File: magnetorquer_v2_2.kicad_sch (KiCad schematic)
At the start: 13 parts, among them U1 MSP430FR5994IPN, Y1 Crystal

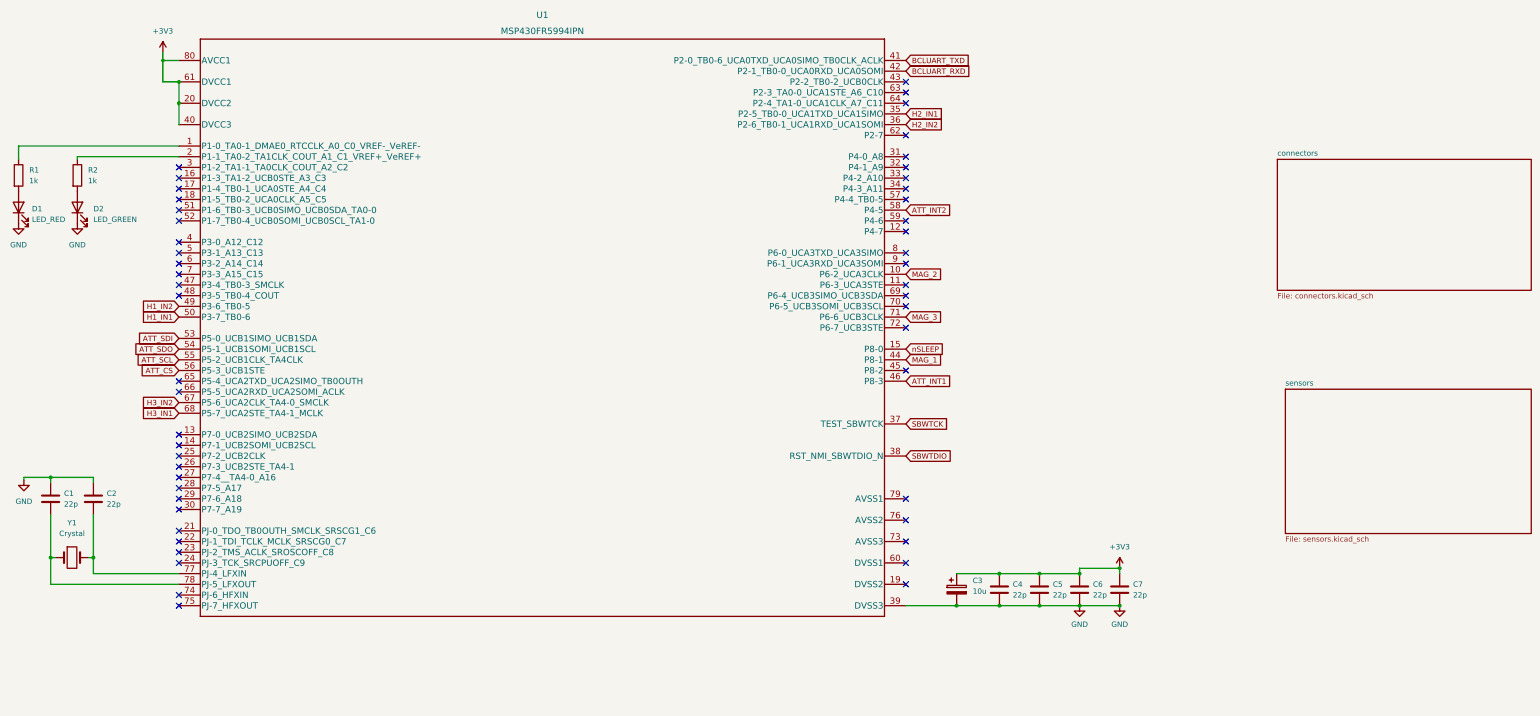
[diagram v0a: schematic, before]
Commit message: new uc
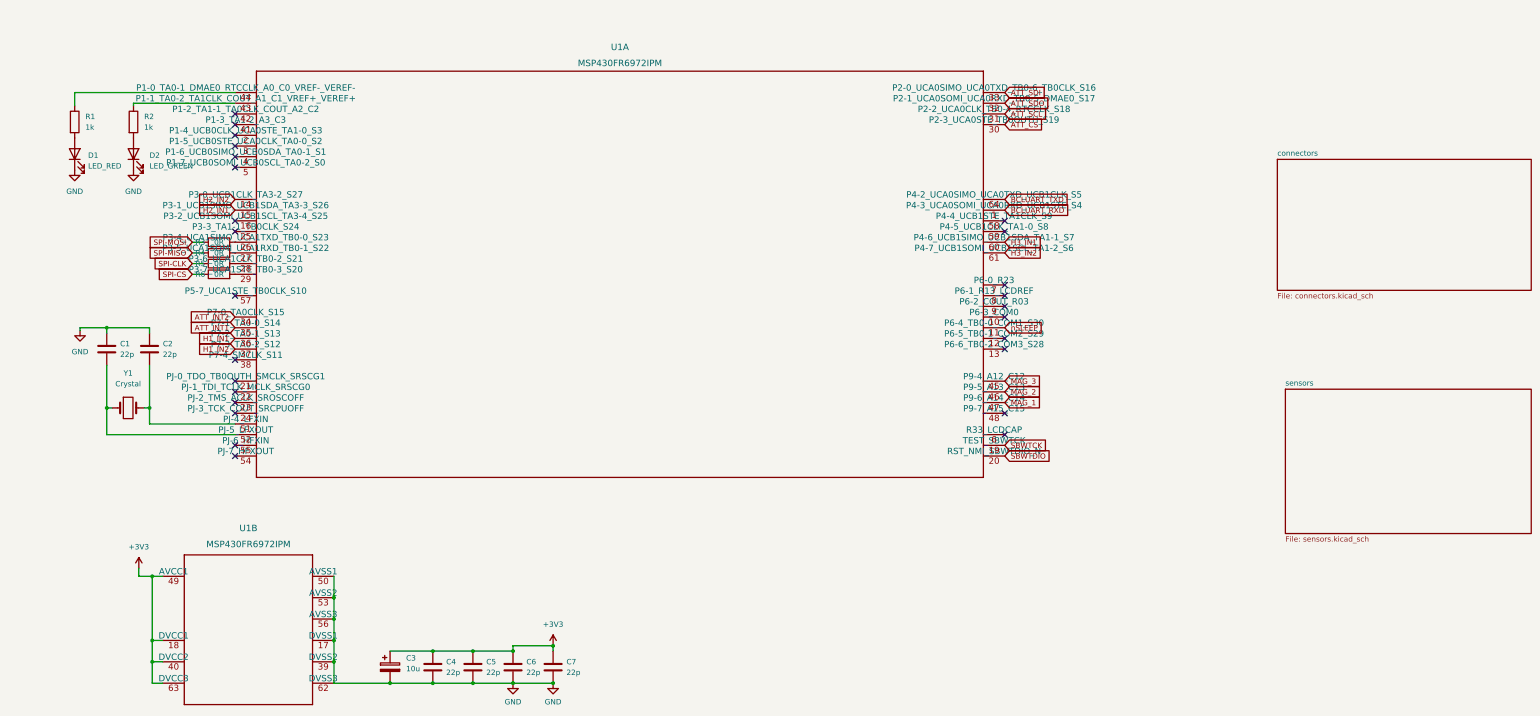
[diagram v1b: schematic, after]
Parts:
- removed U1: MSP430FR5994IPN, magnetorquer:MSP430FR5994IPN, symbol MSP430FR5994IPN:MSP430FR5994IPN
- added R3, R4, R5, R6: 0R, Resistor_SMD:R_0805_2012Metric, symbol Device:R
- added U1: MSP430FR6972IPM, magnetorquer:MSP430FR6972IPM, symbol MSP430FR6972IPM-B:MSP430FR6972IPM
- C3: footprint Capacitor_SMD:C_0805_2012Metric -> Capacitor_Tantalum_SMD:CP_EIA-3216-18_Kemet-A
- D1, D2: footprint LED_SMD:LED_0805_2012Metric -> LED_SMD:LED_0603_1608Metric
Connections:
- net +3V3: now also U1.18 (DVCC1), U1.40 (DVCC2), U1.49 (AVCC1), U1.63 (DVCC3)
- net ATT_CS: now also U1.30 (P2-3_UCA0STE_TB0OUTH_S19)
- net ATT_INT1: now also U1.35 (P7-1_TA0-0_S14)
- net ATT_INT2: now also U1.34 (P7-0_TA0CLK_S15)
- net ATT_SCL: now also U1.31 (P2-2_UCA0CLK_TB0-4_RTCCLK_S18)
- net ATT_SDI: now also U1.33 (P2-0_UCA0SIMO_UCA0TXD_TB0-6_TB0CLK_S16)
- net ATT_SDO: now also U1.32 (P2-1_UCA0SOMI_UCA0RXD_TB0-5_DMAE0_S17)
- net BCLUART_RXD: now also U1.1 (P4-3_UCA0SOMI_UCA0RXD_UCB1STE_S4)
- net BCLUART_TXD: now also U1.64 (P4-2_UCA0SIMO_UCA0TXD_UCB1CLK_S5)
- net GND: now also U1.17 (DVSS1), U1.39 (DVSS2), U1.50 (AVSS1), U1.53 (AVSS2), U1.56 (AVSS3), U1.62 (DVSS3)
- net H1_IN1: now also U1.36 (P7-2_TA0-1_S13)
- net H1_IN2: now also U1.37 (P7-3_TA0-2_S12)
- net H2_IN1: now also U1.15 (P3-1_UCB1SIMO_UCB1SDA_TA3-3_S26)
- net H2_IN2: now also U1.14 (P3-0_UCB1CLK_TA3-2_S27)
- net H3_IN1: now also U1.60 (P4-6_UCB1SIMO_UCB1SDA_TA1-1_S7)
- net H3_IN2: now also U1.61 (P4-7_UCB1SOMI_UCB1SCL_TA1-2_S6)
- net MAG_1: now also U1.47 (P9-6_A14_C14)
- net MAG_2: now also U1.46 (P9-5_A13_C13)
- net MAG_3: now also U1.45 (P9-4_A12_C12)
- net SBWTCK: now also U1.19 (TEST_SBWTCK)
- net SBWTDIO: now also U1.20 (RST_NMI_SBWTDIO_N)
- net nSLEEP: now also U1.11 (P6-4_TB0-0_COM1_S30)
- net at R1.1: now also U1.44 (P1-0_TA0-1_DMAE0_RTCCLK_A0_C0_VREF-_VEREF-)
- net at C1.2, Y1.1: now also U1.52 (PJ-5_LFXOUT)
- net at C2.2, Y1.2: now also U1.51 (PJ-4_LFXIN)
- net at R2.1: now also U1.43 (P1-1_TA0-2_TA1CLK_COUT_A1_C1_VREF+_VEREF+)
- new net: R3.2, U1.26 (P3-4_UCA1SIMO_UCA1TXD_TB0-0_S23)
- new net: R4.2, U1.27 (P3-5_UCA1SOMI_UCA1RXD_TB0-1_S22)
- new net: R5.2, U1.28 (P3-6_UCA1CLK_TB0-2_S21)
- new net: R6.2, U1.29 (P3-7_UCA1STE_TB0-3_S20)
- new net SPI-CLK: R5.1
- new net SPI-CS: R6.1
- new net SPI-MISO: R4.1
- new net SPI-MOSI: R3.1
- no-connect marks 51 -> 26
